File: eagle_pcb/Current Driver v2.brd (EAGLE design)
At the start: 47.9 x 36.8 mm, 12 parts, among them IC1 LM358N, Q2 IRF540

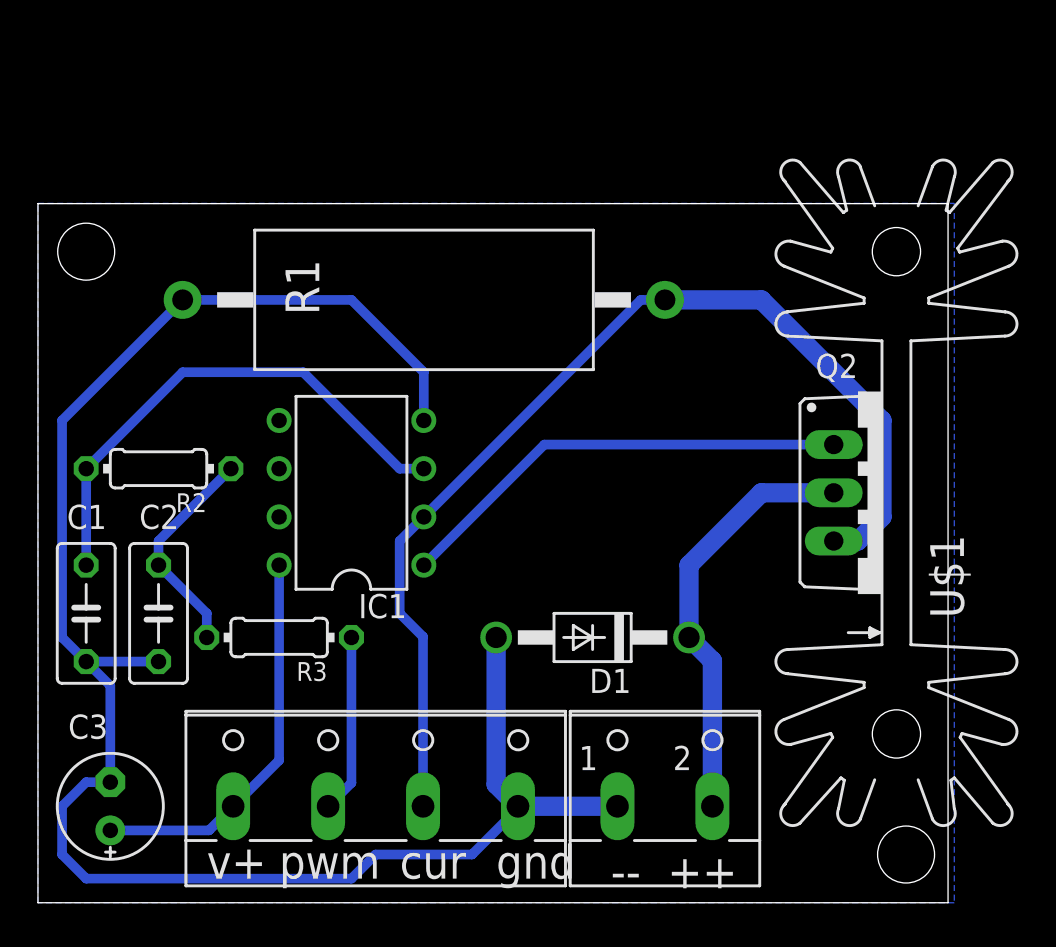
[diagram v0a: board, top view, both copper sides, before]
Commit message: v2
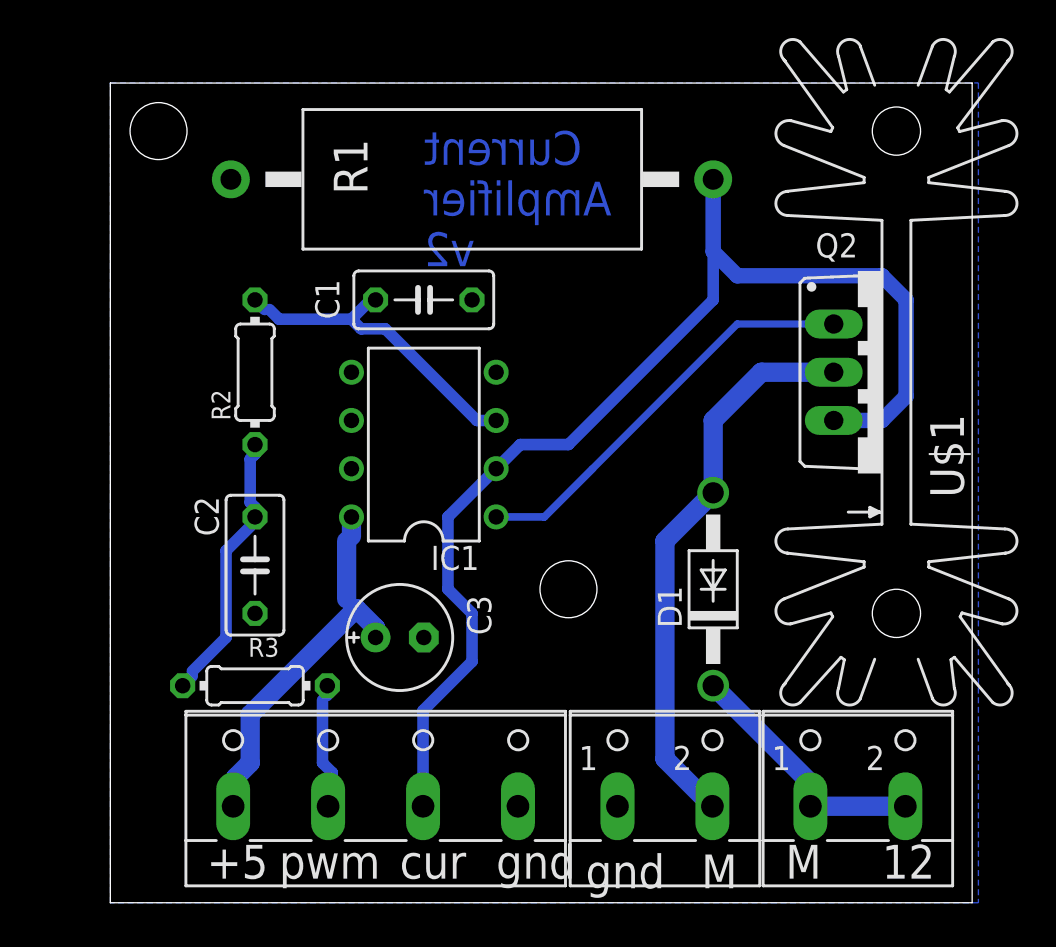
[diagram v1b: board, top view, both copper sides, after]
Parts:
- added X2: (no value), con-wago-500:W237-102
- moved C1 24.3 mm to (24.1, 31.8), turned to 0 degrees
- moved C3 17.6 mm to (22.9, 14.0), turned to 0 degrees
- moved R2 7.18 mm to (15.2, 27.9), turned to 90 degrees
- moved R1 6.84 mm to (26.7, 38.1)
- moved D1 6.84 mm to (39.4, 16.5), turned to 90 degrees
- moved Q2 6.35 mm to (48.3, 27.9)
- moved U$1 6.35 mm to (48.3, 27.9)
- moved C2 5.68 mm to (15.2, 17.8)
- moved IC1 4.58 mm to (24.1, 24.1)
- moved R3 2.84 mm to (15.2, 11.4)
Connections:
- removed net N$3: D1.C, Q2.D, X1.2
- new net N$2: D1.A, Q2.D, X1.2
- new net VSS: D1.C, X2.1, X2.2
- net V-: no longer D1.A
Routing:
- net V-: track 96.3 -> 0.00 mm
- net N$2: track 0.00 -> 29.8 mm
- net N$3: track 22.4 -> 0.00 mm
- net VSS: track 0.00 -> 13.5 mm
- net N$5: track 27.1 -> 17.0 mm
- net N$7: track 55.9 -> 62.5 mm
- net N$1: track 25.5 -> 22.0 mm
- net N$4: track 11.5 -> 14.5 mm
- net N$6: track 9.40 -> 6.88 mm
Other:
- board size 47.9 x 36.8 mm -> 45.4 x 43.2 mm
- board text added: "+5"
- board text added: "12"
- board text added: "Current Amplifier v2"
- board text added: "M"
- board text removed: "++"
- board text removed: "--"
- board text removed: "v+"
